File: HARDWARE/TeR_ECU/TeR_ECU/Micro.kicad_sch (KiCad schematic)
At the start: 1 part, among them U3 STM32F446RETx

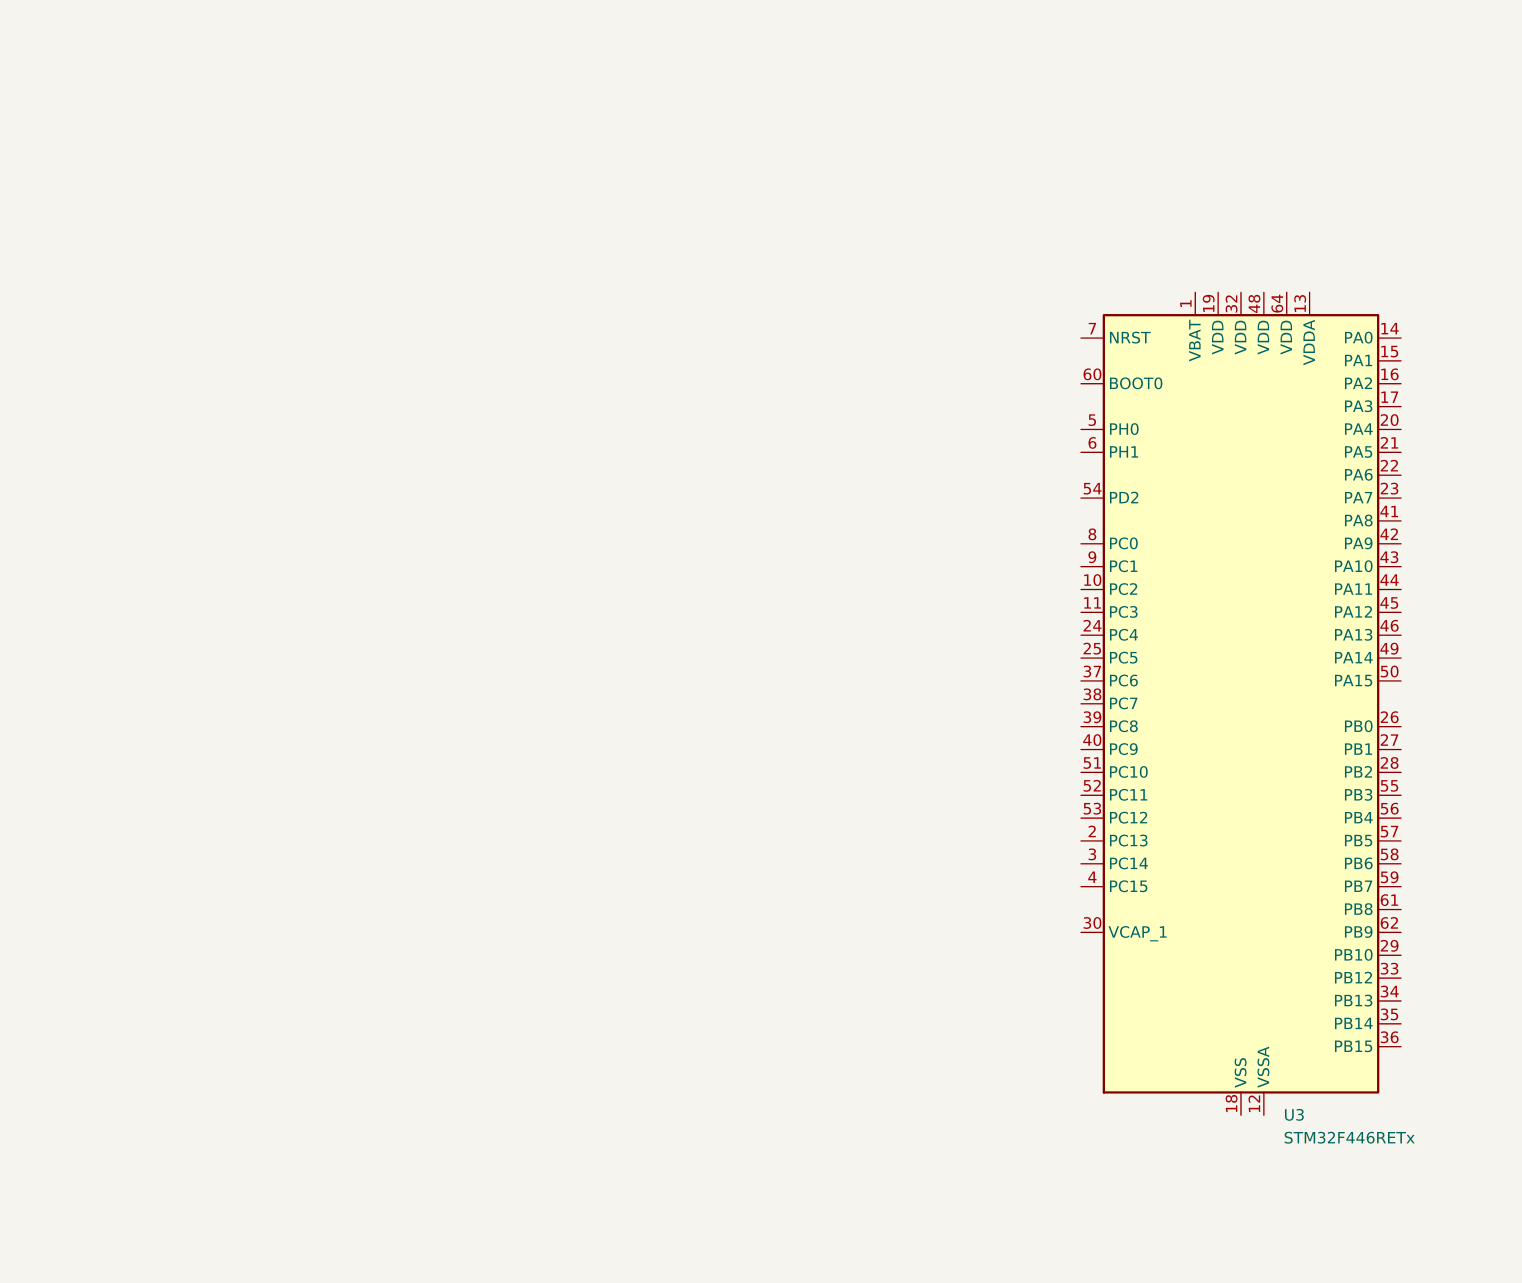
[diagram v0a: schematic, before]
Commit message: Micro
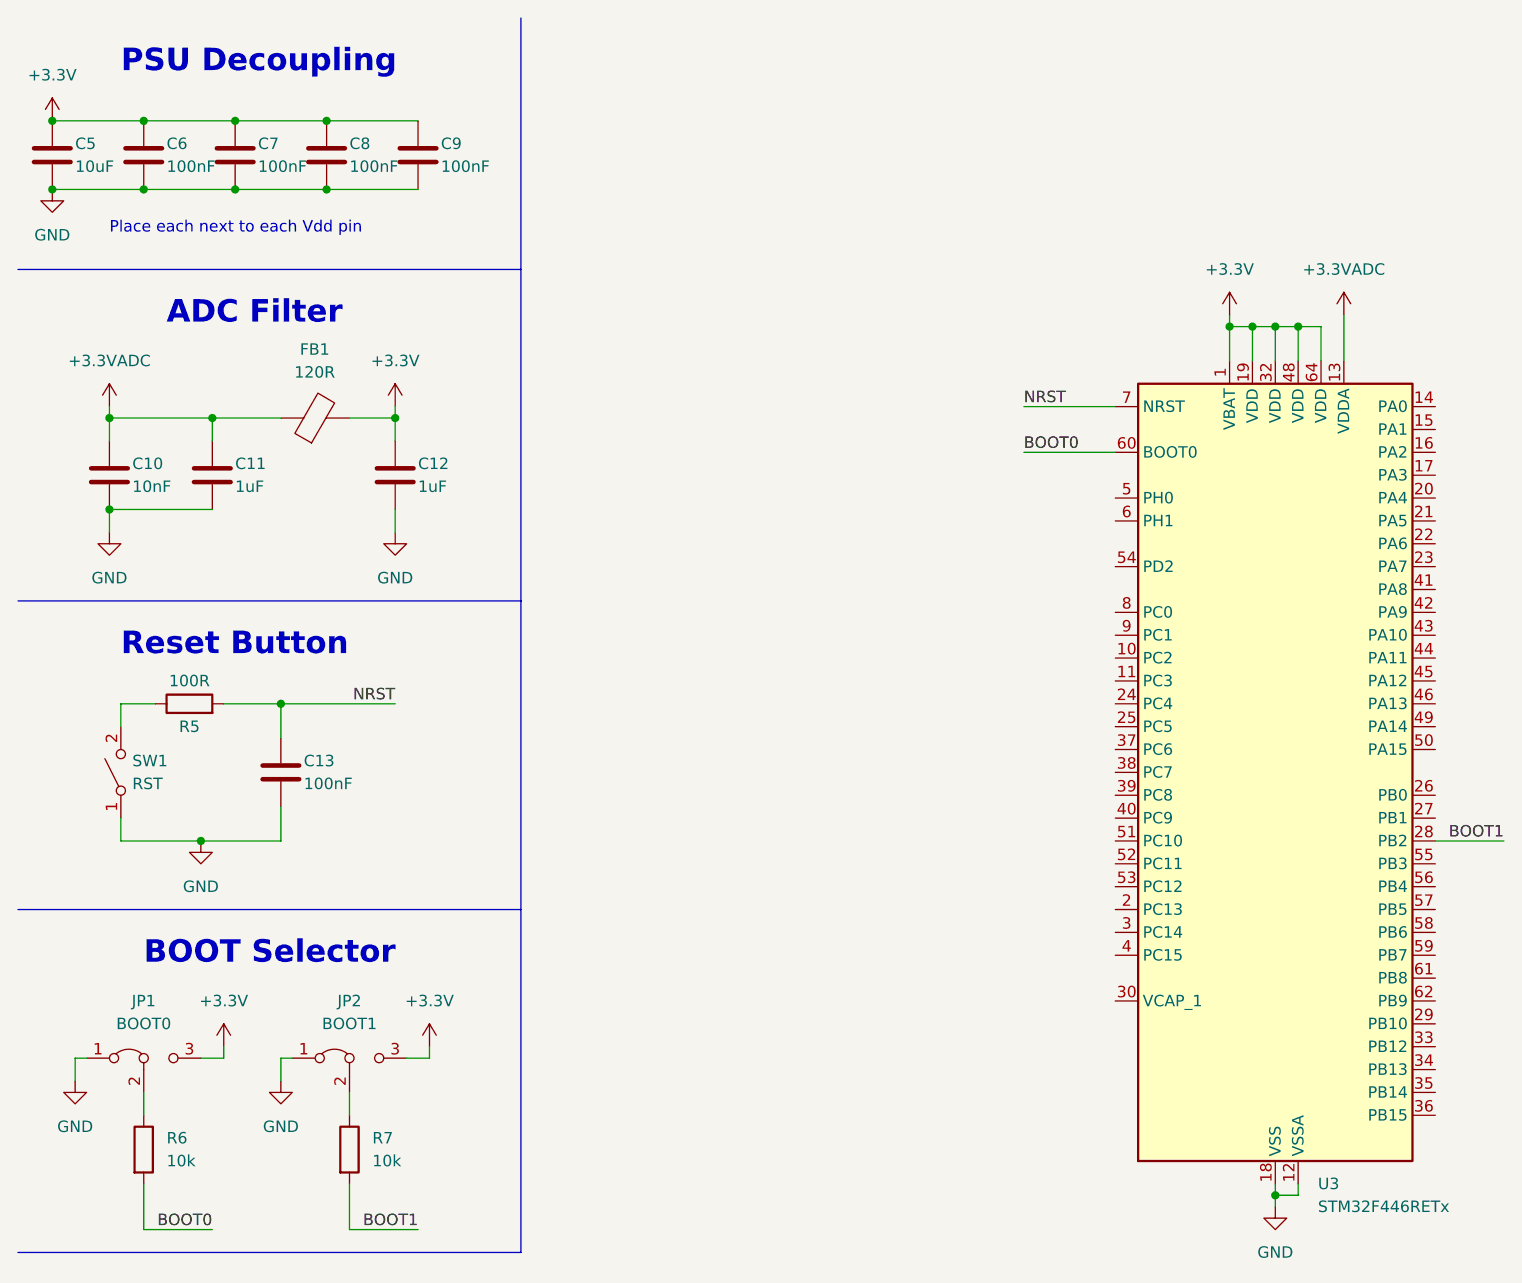
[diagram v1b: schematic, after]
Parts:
- added C10: 10nF, Capacitor_SMD:C_0805_2012Metric, symbol Device:C
- added C11, C12: 1uF, Capacitor_SMD:C_0805_2012Metric, symbol Device:C
- added C13, C6, C7, C8, C9: 100nF, Capacitor_SMD:C_0805_2012Metric, symbol Device:C
- added C5: 10uF, Capacitor_SMD:C_0805_2012Metric, symbol Device:C
- added FB1: 120R, symbol Device:FerriteBead
- added JP1: BOOT0, symbol Jumper:Jumper_3_Bridged12
- added JP2: BOOT1, symbol Jumper:Jumper_3_Bridged12
- added R5: 100R, symbol Device:R
- added R6, R7: 10k, symbol Device:R
- added SW1: RST, symbol Switch:SW_SPST
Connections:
- net +3.3V: now reaches U3.1 (VBAT)
- net +3.3V: now also U3.19 (VDD), U3.32 (VDD), U3.48 (VDD), U3.64 (VDD), C12.2, C5.2, C6.2, C7.2, C8.2, C9.2, FB1.2, JP1.3 (B), JP2.3 (B)
- net GND: now reaches U3.12 (VSSA)
- net GND: now also U3.18 (VSS), U3.31 (VSS), U3.47 (VSS), U3.63 (VSS), C10.1, C11.1, C12.1, C13.1, C5.1, C6.1, C7.1, C8.1, C9.1, JP1.1 (A), JP2.1 (A), SW1.1 (A)
- net +3.3VADC: now reaches U3.13 (VDDA)
- net +3.3VADC: now also C10.2, C11.2, FB1.1
- net BOOT1: now reaches U3.28 (PB2)
- net BOOT1: now also R7.2
- net BOOT0: now reaches U3.60 (BOOT0)
- net BOOT0: now also R6.2
- net NRST: now reaches U3.7 (NRST)
- net NRST: now also C13.2, R5.2
- new net: JP1.2 (C), R6.1
- new net: R5.1, SW1.2 (B)
- new net: JP2.2 (C), R7.1
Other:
- note added: "ADC Filter"
- note added: "BOOT Selector"
- note added: "PSU Decoupling"
- note added: "Place each next to each Vdd pin"
- note added: "Reset Button"
- moved on the sheet: U3
